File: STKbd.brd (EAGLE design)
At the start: 189.6 x 80.6 mm, 70 parts, among them IC1 MEGA8-AI, IC2 DS1813-SMD, Q1 20 MHz, X1 MKDSN1,5/2-5,08, X2 MKDSN1,5/2-5,08, X3 MKDSN1,5/2-5,08, X4 22-23-2021, X5 MKDSN1,5/2-5,08, X6 MKDSN1,5/2-5,08, X7 MKDSN1,5/2-5,08

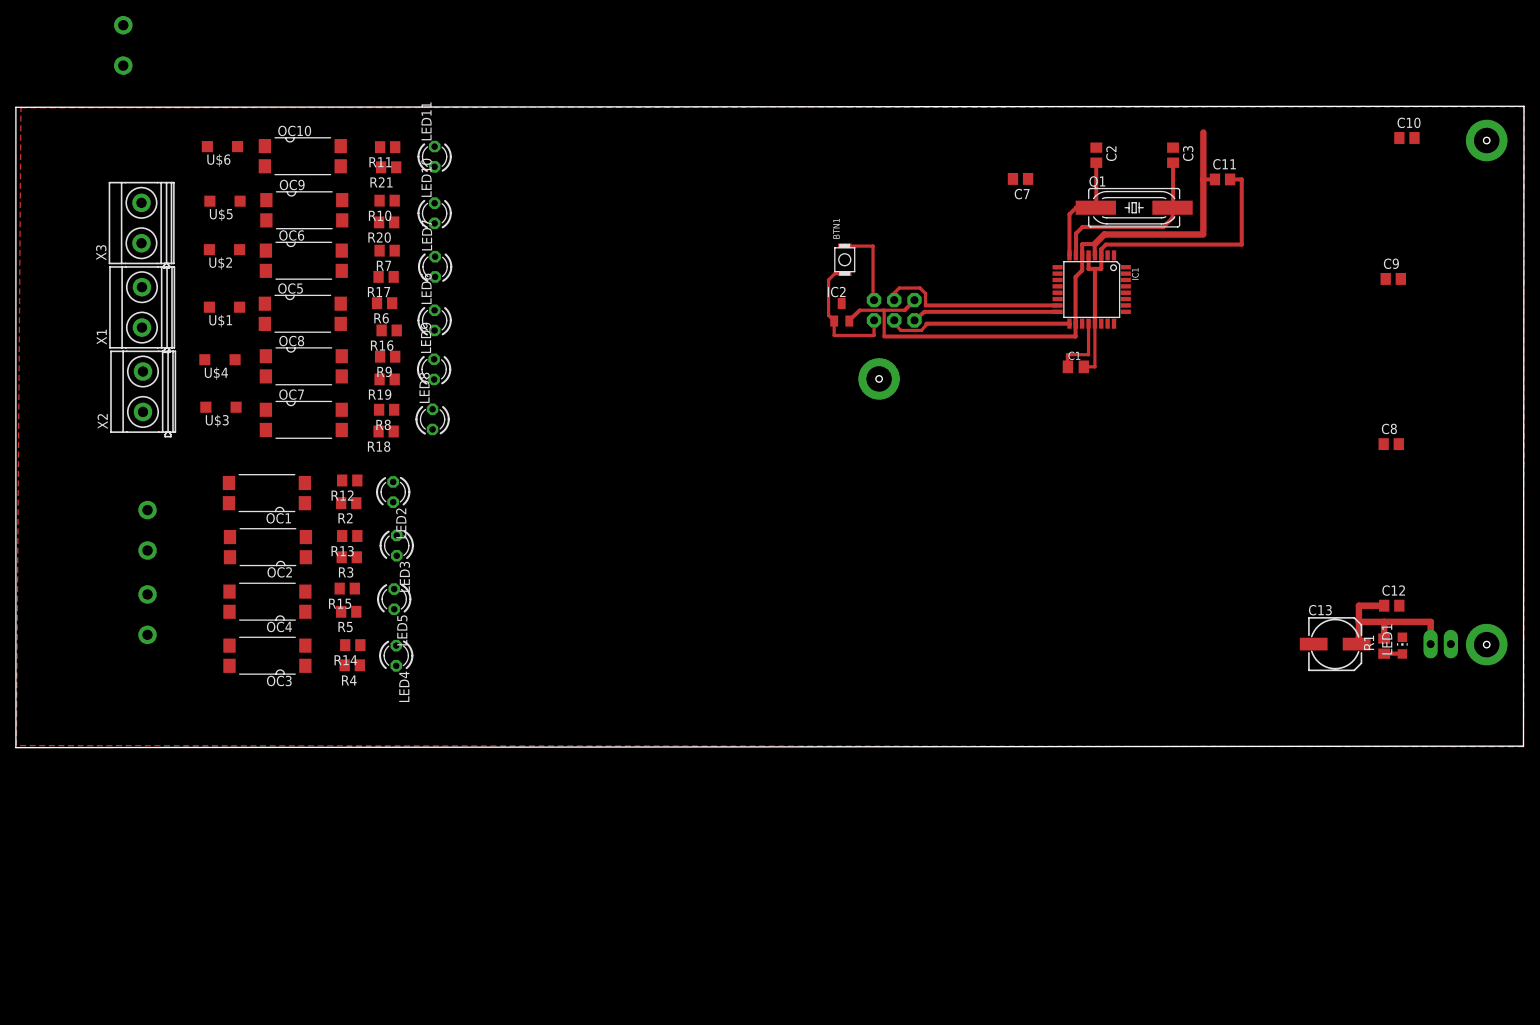
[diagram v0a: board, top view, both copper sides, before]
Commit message: Rev 1.0
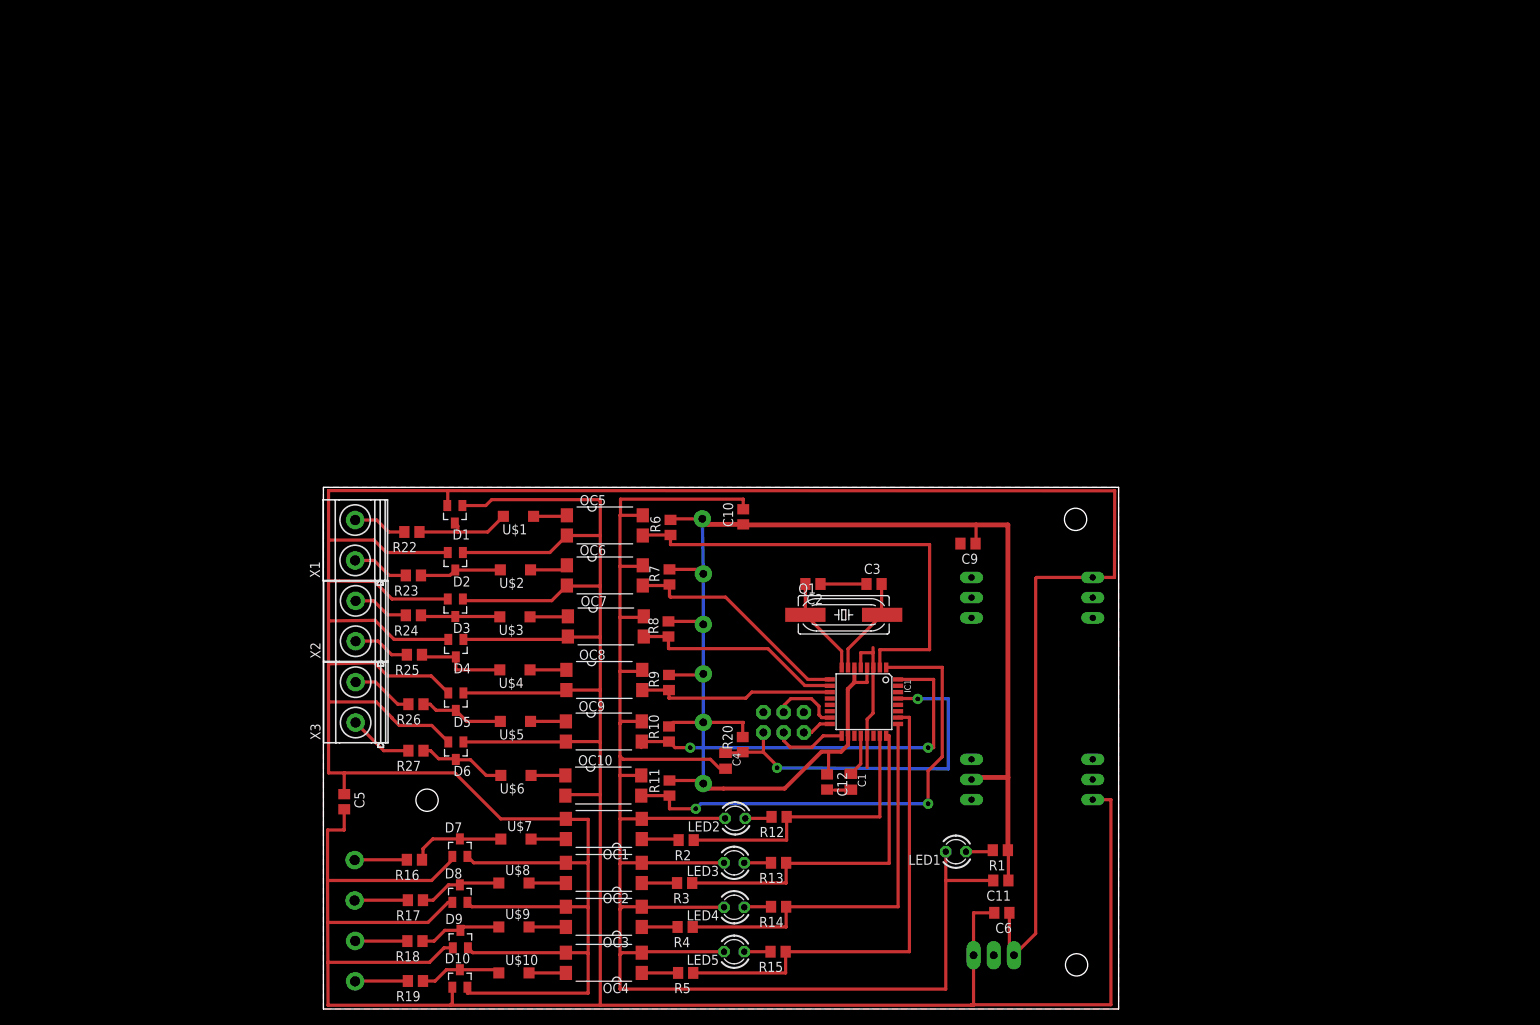
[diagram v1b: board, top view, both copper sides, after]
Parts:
- removed BTN1: SPST.B3U-1000P(M), omron:B3U-1000P(M)
- removed C13: (no value), rcl:153CLV-0605
- removed C7, C8: (no value), rcl:C0805
- removed IC2: DS1813-SMD, ds1813_revised:SOT-23
- removed LED10, LED11, LED6, LED7, LED8, LED9: LED, MyLib:LED3MM
- removed R21: 1k, rcl:R0805
- removed X4: 22-23-2021, con-molex:22-23-2021
- added C4: 0.1u, rcl:C0805K
- added C5, C6: (no value), rcl:C0805
- added D1, D10, D2, D3, D4, D5, D6, D7, D8, D9: BAV199, diode:SOT23
- added R22, R23, R24, R25, R26, R27: 50R, rcl:R0805
- added U$10, U$7, U$8, U$9: NSI45020AT1GSOD-123, MyLib:SOD123
- added U$11: TRACO_TEL_3-2411, MyLib:TEL-3
- LED1: value (none) -> LED; device led:CHIP-LED0805 -> MyLib:LED3MM
- R10, R11, R7, R8, R9: value 50R -> 1k
- R16, R17, R18, R19: value 1k -> 50R
- R20: value 1k -> 10k
- X7: value MKDSN1,5/2-5,08 -> 22-23-2031; device con-phoenix-508:MKDSN1,5/2-5,08 -> con-molex:22-23-2031
- moved X7 158.3 mm to (34.3, -26.0), turned to 0 degrees
- moved C10 96.1 mm to (2.79, 29.1), turned to 90 degrees
- moved C11 92.4 mm to (35.2, -16.6), turned to 180 degrees
- moved R11 88.0 mm to (-6.48, -5.02), turned to 90 degrees
- moved OC10 87.7 mm to (-14.8, -4.70)
- moved U$6 87.2 mm to (-25.8, -3.43)
- moved R20 79.5 mm to (2.73, 0.44), turned to 90 degrees
- moved R17 78.4 mm to (-38.4, -19.1)
- moved R10 75.8 mm to (-6.54, 1.78), turned to 90 degrees
- moved R19 75.7 mm to (-38.4, -29.3)
- moved OC9 75.6 mm to (-14.7, 2.10)
- moved U$5 74.9 mm to (-25.8, 3.37)
- moved C12 74.4 mm to (13.3, -4.25), turned to 270 degrees
- moved R15 70.8 mm to (7.18, -25.6)
- moved R12 68.6 mm to (7.30, -8.64)
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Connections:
- removed net N$31 (its old number): LED9.A, R19.1
- removed net N$32 (its old number): LED10.A, R20.1
- removed net N$33 (its old number): LED11.A, R21.1
- removed net N$68: LED1.A, R1.1
- removed net N$76: IC1.19
- new net N$17: D9.3, R18.1, U$9.C
- new net N$18: R18.2, X6.1
- new net N$19: D10.3, R19.1, U$10.C
- new net N$20: R19.2, X6.2
- new net N$34: OC1.4, U$7.A
- new net N$38: D3.3, R24.1, U$3.A
- new net N$39: D1.3, R22.1, U$1.A
- new net N$40: D4.3, R25.1, U$4.A
- new net N$41: D5.3, R26.1, U$5.A
- new net N$42: D6.3, R27.1, U$6.A
- new net N$43: R27.2, X3.1
- new net N$44: LED1.A, R1.2
- net +24V: now also C5.1, C6.1, D1.2, D10.2, D2.2, D3.2, D4.2, D5.2, D6.2, D7.2, D8.2, D9.2, U$11.1, U$11.24
- net +5V: now also R1.1, R10.2, R11.2, R20.2, R6.2, R7.2, R8.2, R9.2, U$11.11, U$11.14; no longer C13.+, C7.1, C8.1, IC2.2, OC10.3, OC5.3, OC6.3, OC7.3, OC8.3, OC9.3, R1.2, X4.1
- net GND: now also C4.2, LED1.K, OC10.4, OC5.4, OC6.4, OC7.4, OC8.4, OC9.4, U$11.10, U$11.15; no longer BTN1.2, C13.-, C7.2, C8.2, IC2.3, LED1.C, LED10.K, LED11.K, LED6.K, LED7.K, LED8.K, LED9.K, R10.1, R11.1, R6.1, R7.1, R8.1, R9.1, X4.2
- net K1: now also OC5.3, R6.1; no longer OC5.4, R16.2, R6.2
- net K2: now also OC6.3, R7.1; no longer OC6.4, R17.2, R7.2
- net K3: now also OC7.3, R8.1; no longer OC7.4, R18.2, R8.2
- net K4: now also OC8.3, R9.1; no longer OC8.4, R19.2, R9.2
- net N$10: now also D7.3, R16.1, U$7.C; no longer OC1.4, X5.1
- net N$11: now also D8.3, R17.1, U$8.C; no longer OC2.4, X5.2
- net N$13: now also R16.2, X5.1; no longer OC3.4, X6.2
- net N$14: now also R17.2, X5.2; no longer OC4.4, X6.1
- net N$22: now also R22.2; no longer U$2.A
- net N$24: now also R26.2, X3.2; no longer U$4.A, X2.2
- net N$25: now also R23.2, X1.1; no longer U$5.A, X3.1
- net N$26: now also R25.2, X2.1; no longer U$6.A, X3.2
- net N$28: now also OC4.4, U$10.A; no longer LED6.A, R16.1
- net N$29: now also OC3.4, U$9.A; no longer LED7.A, R17.1
- net N$30: now also OC2.4, U$8.A; no longer LED8.A, R18.1
- net N$8: now also R24.2, X2.2; no longer U$3.A, X2.1
- net N$9: now also D2.3, R23.1, U$2.A; no longer U$1.A, X1.1
- net PE: now also C5.2, C6.2, D1.1, D10.1, D2.1, D3.1, D4.1, D5.1, D6.1, D7.1, D8.1, D9.1, U$11.12, U$11.13, X7.3; no longer X7.2
- net RESET: now also C4.1, R20.1; no longer BTN1.1, IC2.1
- net RS1: now also OC9.3, R10.1; no longer OC9.4, R10.2, R20.2
- net RS2: now also OC10.3, R11.1; no longer OC10.4, R11.2, R21.2
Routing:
- net +24V: track 0.00 -> 415.8 mm
- net PE: track 0.00 -> 395.2 mm
- net GND: track 57.8 -> 252.1 mm, vias 3 -> 0
- net +5V: track 102.8 -> 196.8 mm, vias 0 -> 6
- net RS2: track 0.00 -> 63.1 mm, vias 0 -> 2
- net S4: track 0.00 -> 60.8 mm
- net K1: track 0.00 -> 59.1 mm
- net S3: track 0.00 -> 51.3 mm
- net RS1: track 0.00 -> 50.9 mm, vias 0 -> 2
- net S2: track 0.00 -> 43.8 mm
- net S1: track 0.00 -> 36.6 mm
- net RESET: track 16.6 -> 46.7 mm, vias 0 -> 2
- net K2: track 0.22 -> 29.7 mm
- net K3: track 0.00 -> 26.8 mm
- net K4: track 0.00 -> 24.9 mm
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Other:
- board size 189.6 x 80.6 mm -> 100 x 65.6 mm
